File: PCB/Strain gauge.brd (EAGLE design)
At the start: 69.5 x 69.8 mm, 11 parts

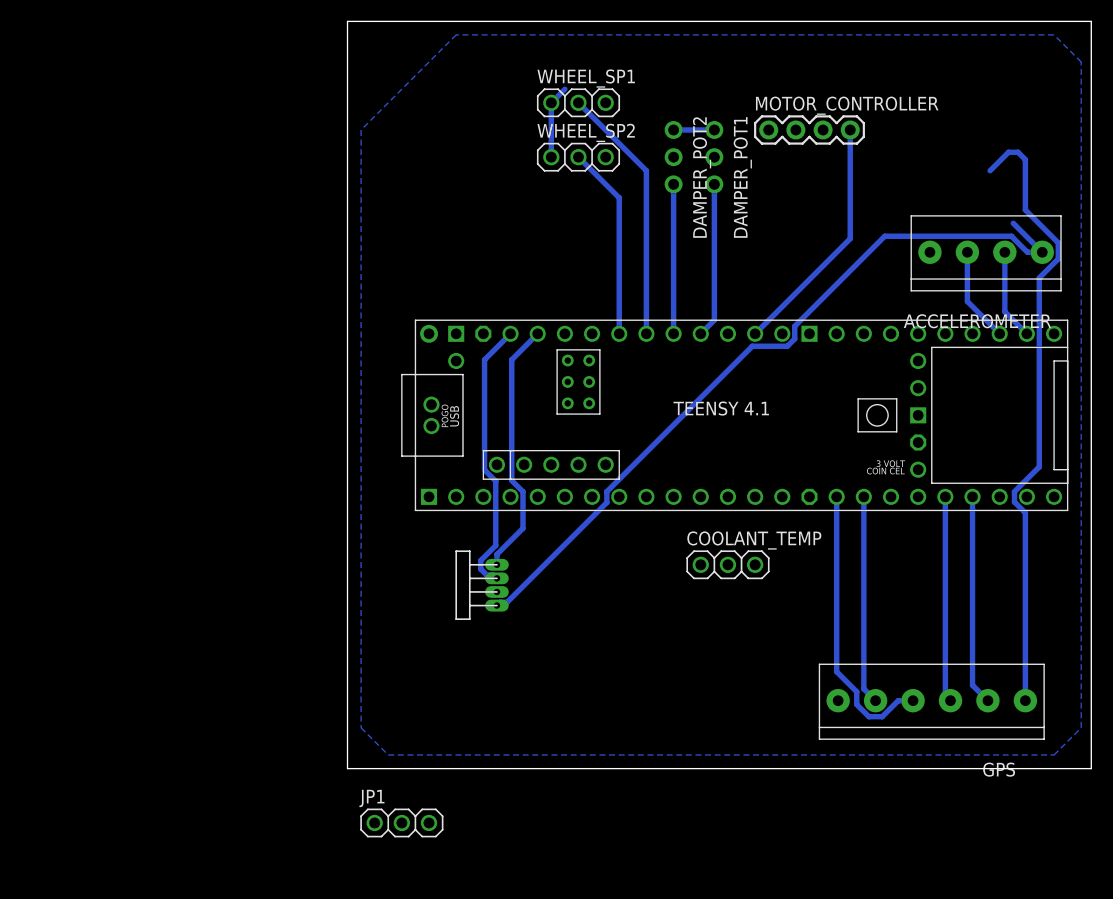
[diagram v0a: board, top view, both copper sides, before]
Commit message: Updated ECU and Strain Gauge board
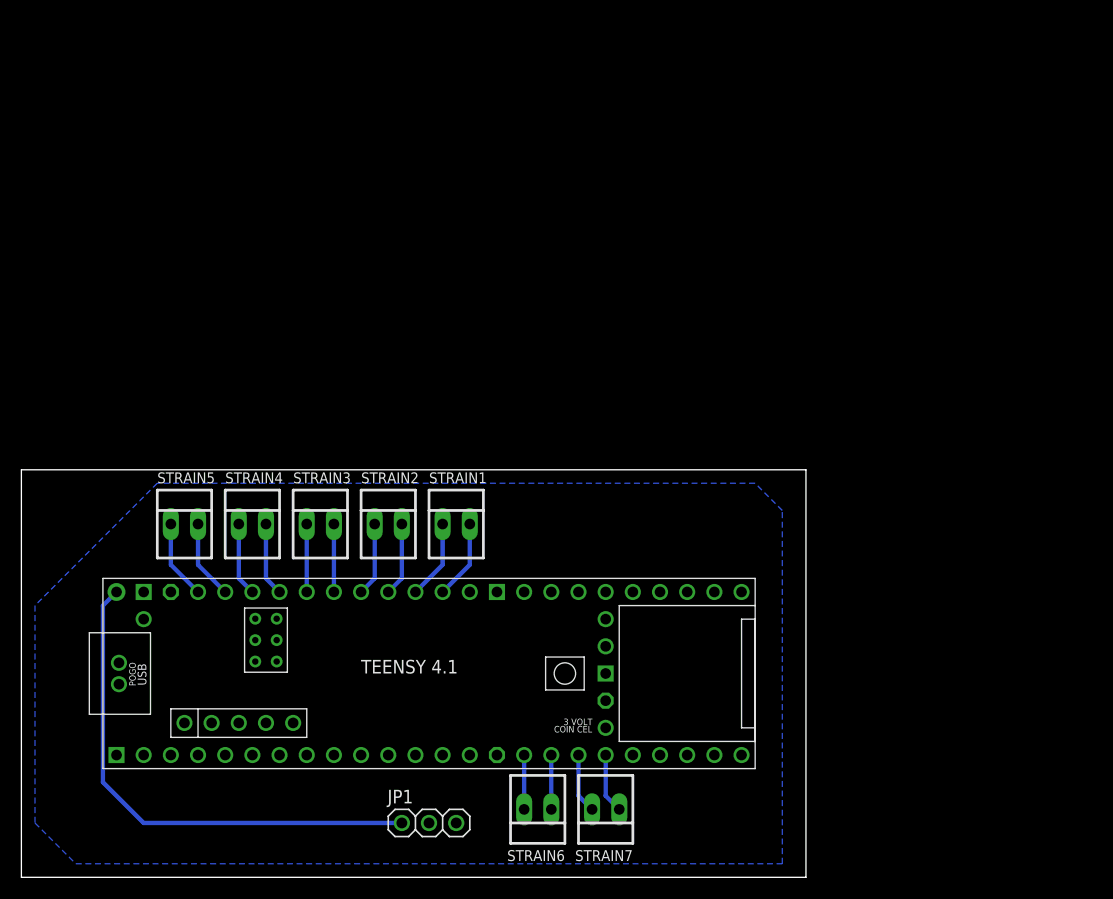
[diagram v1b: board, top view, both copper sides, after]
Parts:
- removed ACCELEROMETER: 1X4-3.5MM, adafruit:1X04-3.5MM
- removed CAN1_TEE: CAN_TEE, F-E library custom components:CAN_TEN
- removed COOLANT_TEMP, WHEEL_SP1, WHEEL_SP2: (no value), adafruit:1X03
- removed DAMPER_POT1, DAMPER_POT2: (no value), adafruit:1X03-CLEANBIG
- removed GPS: (no value), adafruit:1X06-3.5MM
- removed MOTOR_CONTROLLER: 1X4-BIG, adafruit:1X04-BIG
- added STRAIN1, STRAIN2, STRAIN3, STRAIN4, STRAIN5, STRAIN6, STRAIN7: 22-23-2021, con-molex:22-23-2021
- moved U$1 37.9 mm to (39.4, 19.1)
- moved JP1 2.54 mm to (38.1, 5.08)
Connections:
- removed net 3.3V: ACCELEROMETER.4, CAN1_TEE.P$1, U$1.3V3-1
- removed net A2: DAMPER_POT1.3, U$1.16-A2/RX4/SCL1
- removed net A3: DAMPER_POT2.3, U$1.17-A3/TX4/SDA1
- removed net A_MC: MOTOR_CONTROLLER.4, U$1.14-A0/TX3/SPDIF_OUT
- removed net BR_VCC: DAMPER_POT1.1, DAMPER_POT2.1
- removed net RX: ACCELEROMETER.2, U$1.35-TX8
- removed net RX_2: GPS.5, U$1.29-TX7
- removed net SCL: GPS.3, U$1.24-A10/TX6/SCL2
- removed net SDA: GPS.2, U$1.25-A11/RX6/SDA2
- removed net TX: ACCELEROMETER.3, U$1.34-RX8
- removed net TX_2: GPS.4, U$1.28-RX7
- removed net WH_SP1_D: U$1.18-A4/SDA0, WHEEL_SP1.2
- removed net WH_SP2_D: U$1.19-A5/SCL0, WHEEL_SP2.2
- new net N$1: STRAIN1.2, U$1.14-A0/TX3/SPDIF_OUT
- new net N$10: STRAIN5.1, U$1.23-A9/CRX1/MCLK1
- new net N$11: STRAIN6.2, U$1.24-A10/TX6/SCL2
- new net N$12: STRAIN6.1, U$1.25-A11/RX6/SDA2
- new net N$13: STRAIN7.2, U$1.26-A12/MOSI1
- new net N$14: STRAIN7.1, U$1.27-A13/SCK1
- new net N$4: STRAIN2.1, U$1.17-A3/TX4/SDA1
- new net N$5: STRAIN3.2, U$1.18-A4/SDA0
- new net N$6: STRAIN3.1, U$1.19-A5/SCL0
- new net N$7: STRAIN4.2, U$1.20-A6/TX5/LRCLK1
- new net N$8: STRAIN4.1, U$1.21-A7/RX5/BCLK1
- new net N$9: STRAIN5.2, U$1.22-A8/CTX1
- net 12V: now also JP1.2; no longer JP1.3, WHEEL_SP1.1, WHEEL_SP2.1
- net 5V: now also JP1.1; no longer GPS.6, JP1.2
- net GND: now also JP1.3; no longer ACCELEROMETER.1, CAN1_TEE.P$2, COOLANT_TEMP.3, DAMPER_POT1.2, DAMPER_POT2.2, GPS.1, JP1.1, MOTOR_CONTROLLER.1, WHEEL_SP1.3, WHEEL_SP2.3
- net N$2: now also STRAIN1.1, U$1.15-A1/RX3/SPDIF_IN; no longer CAN1_TEE.P$3, U$1.23-A9/CRX1/MCLK1
- net N$3: now also STRAIN2.2, U$1.16-A2/RX4/SCL1; no longer CAN1_TEE.P$4, U$1.22-A8/CTX1
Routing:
- net 3.3V: track 71.0 -> 0.00 mm
- net SCL: track 26.5 -> 0.00 mm
- net WH_SP1_D: track 24.2 -> 0.00 mm
- net A_MC: track 22.7 -> 0.00 mm
- net RX_2: track 19.6 -> 0.00 mm
- net SDA: track 19.5 -> 0.00 mm
- net TX_2: track 19.2 -> 0.00 mm
- net N$2: track 25.9 -> 7.40 mm
- net WH_SP2_D: track 18.1 -> 0.00 mm
- net N$3: track 24.0 -> 6.88 mm
- net A2: track 14.5 -> 0.00 mm
- net A3: track 14.0 -> 0.00 mm
- net 5V: track 58.3 -> 47.8 mm
- net RX: track 8.87 -> 0.00 mm
- net TX: track 8.47 -> 0.00 mm
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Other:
- board size 69.5 x 69.8 mm -> 73.3 x 38.1 mm
